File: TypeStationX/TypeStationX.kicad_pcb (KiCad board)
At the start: 2 copper layers, 275.7 x 117 mm, 75 parts, among them J1 Conn_01x09, J2 Conn_01x09, U2 Elite-C

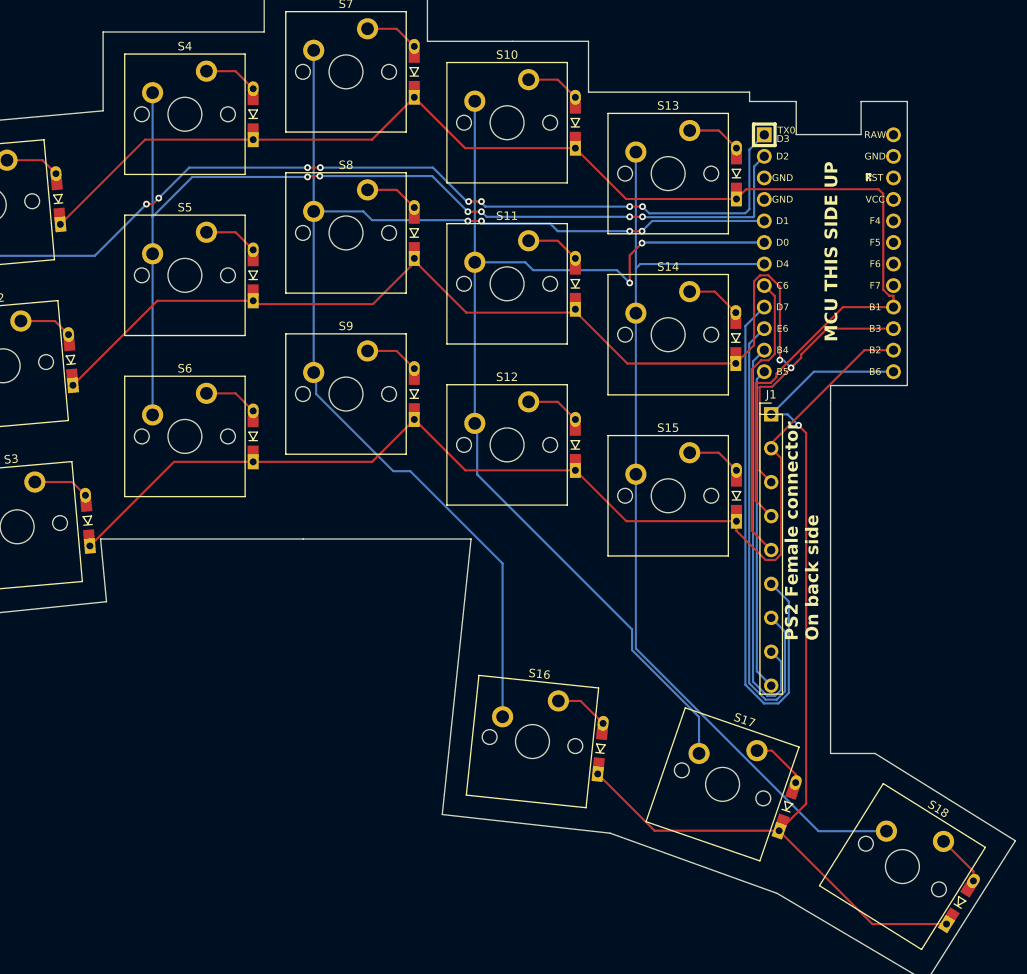
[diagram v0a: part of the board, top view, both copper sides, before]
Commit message: Add files via upload
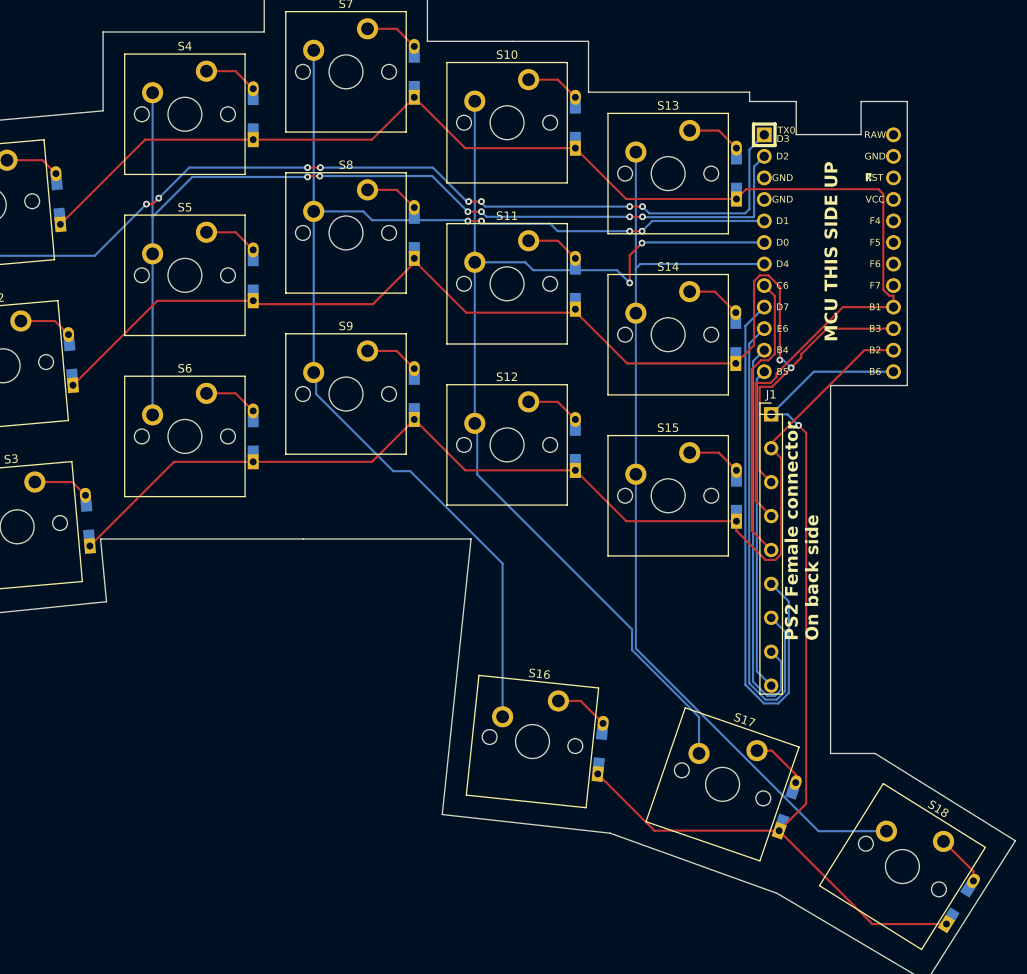
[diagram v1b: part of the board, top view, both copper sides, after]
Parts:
- D1, D10, D11, D12, D13, D14, D15, D16, D17, D18, D2, D3, D4, D5, D6, D7, D8, D9: moved to B.Cu
